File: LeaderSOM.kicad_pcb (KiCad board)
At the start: 4 copper layers, 61 x 50 mm, 108 parts, among them IC1 LP5912-3.3DRVR, IC2 TPS1120DR, J1 SWD, J10 SOMConnector, J11 CAN_Int, J2 USB_B_Micro, J4 Micro_SD_Card_Det, J5 CAN_In2, J6 CAN_Out2, J7 CarPowerConnector, J9 SOMConnector, Q1 PBSS4330X,135, Q2 SI7149ADP-T1-GE3, Q3 SI7149ADP-T1-GE3, SW1 Reset, SW2 BTN1, U1 MAX16914AUB/V+T, U3 CP2102N-A02-GQFN24, U4 ISO1044BD, U5 CDSOT23-T24CAN, U6 STM32F413RHTx, U8 ISO1044BD, U9 CDSOT23-T24CAN, Y2 8M

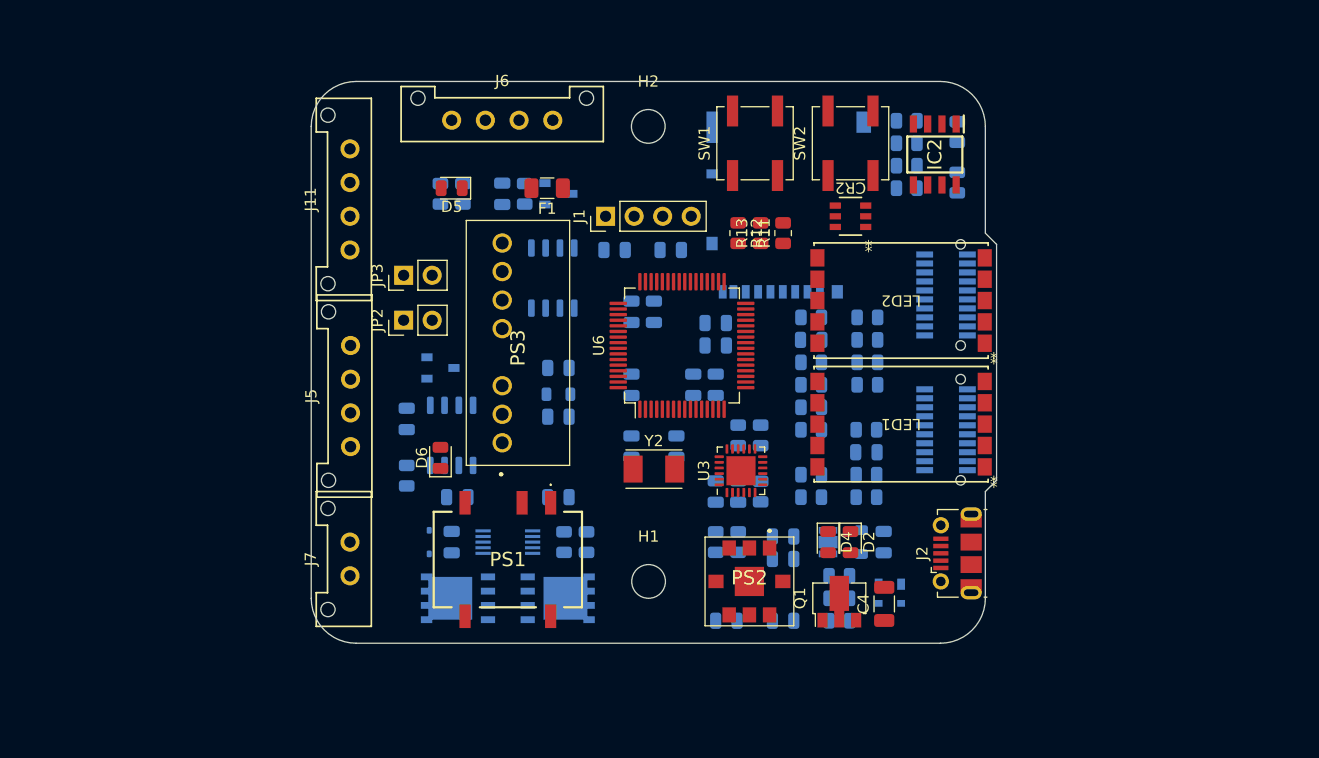
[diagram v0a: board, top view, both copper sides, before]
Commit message: hi lakshay
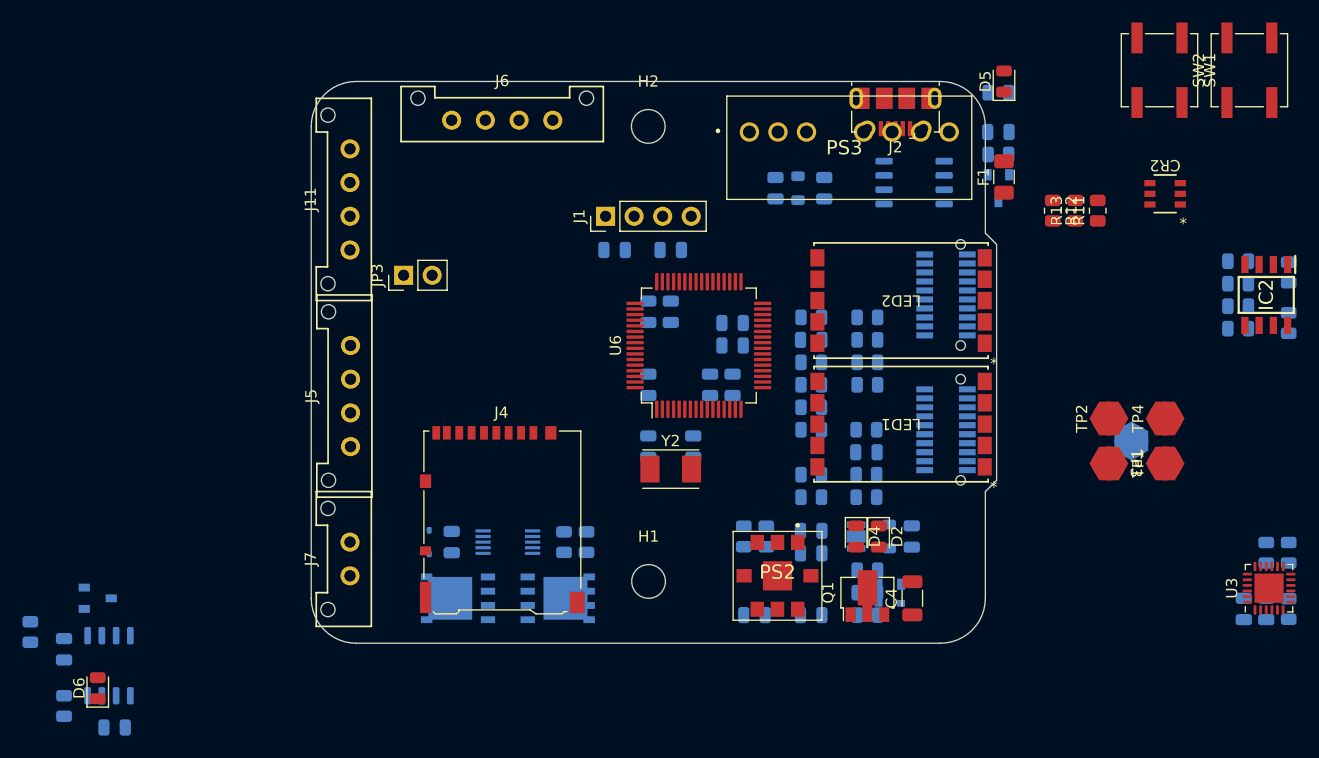
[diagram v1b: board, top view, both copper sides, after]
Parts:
- removed C3: 10uF, Capacitor_SMD:C_0805_2012Metric
- removed JP2: CAN_PWR Jumper, Connector_PinHeader_2.54mm:PinHeader_1x02_P2.54mm_Vertical
- removed PS1: 1769405141, UTSVT_Power:1769405141
- added TP1: +12V_TP, UTSVT_Special:TestPoint_HEX_3mmID, F.Cu at (166.0, 83.0)
- added TP2: +3V3_TP, UTSVT_Special:TestPoint_HEX_3mmID, F.Cu at (161.0, 79.0)
- added TP3: +5V_TP, UTSVT_Special:TestPoint_HEX_3mmID, F.Cu at (161.0, 83.0)
- added TP4: GND_TP, UTSVT_Special:TestPoint_HEX_3mmID, F.Cu at (166.0, 79.0)
- added TP6: GND_TP, UTSVT_Special:TestPoint_HEX_3mmID, B.Cu at (163.0, 81.0)
- J4: moved to F.Cu
- moved R22 53.4 mm to (65.0, 98.0)
- moved D5 50.1 mm to (151.7, 49.0), turned to 90 degrees
- moved R34 48.5 mm to (151.2, 50.0), turned to 180 degrees
- moved C18 48.1 mm to (173.0, 96.0)
- moved C19 48.1 mm to (175.0, 96.0)
- moved R5 48.1 mm to (177.0, 91.0)
- moved R6 48.1 mm to (175.0, 91.0)
- moved R8 48.1 mm to (177.0, 96.0)
- moved U3 48.1 mm to (175.2, 94.1)
- moved C10 44.5 mm to (151.2, 53.5), turned to 180 degrees
- moved R10 42.3 mm to (151.2, 55.5), turned to 180 degrees
- moved F1 40.7 mm to (151.7, 57.5), turned to 90 degrees
- moved J2 39.6 mm to (142.0, 51.7), turned to 180 degrees
- moved U5 39.2 mm to (151.2, 58.5), turned to -90 degrees
- moved J4 37.9 mm to (107.0, 88.0)
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
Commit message: u is for u n me
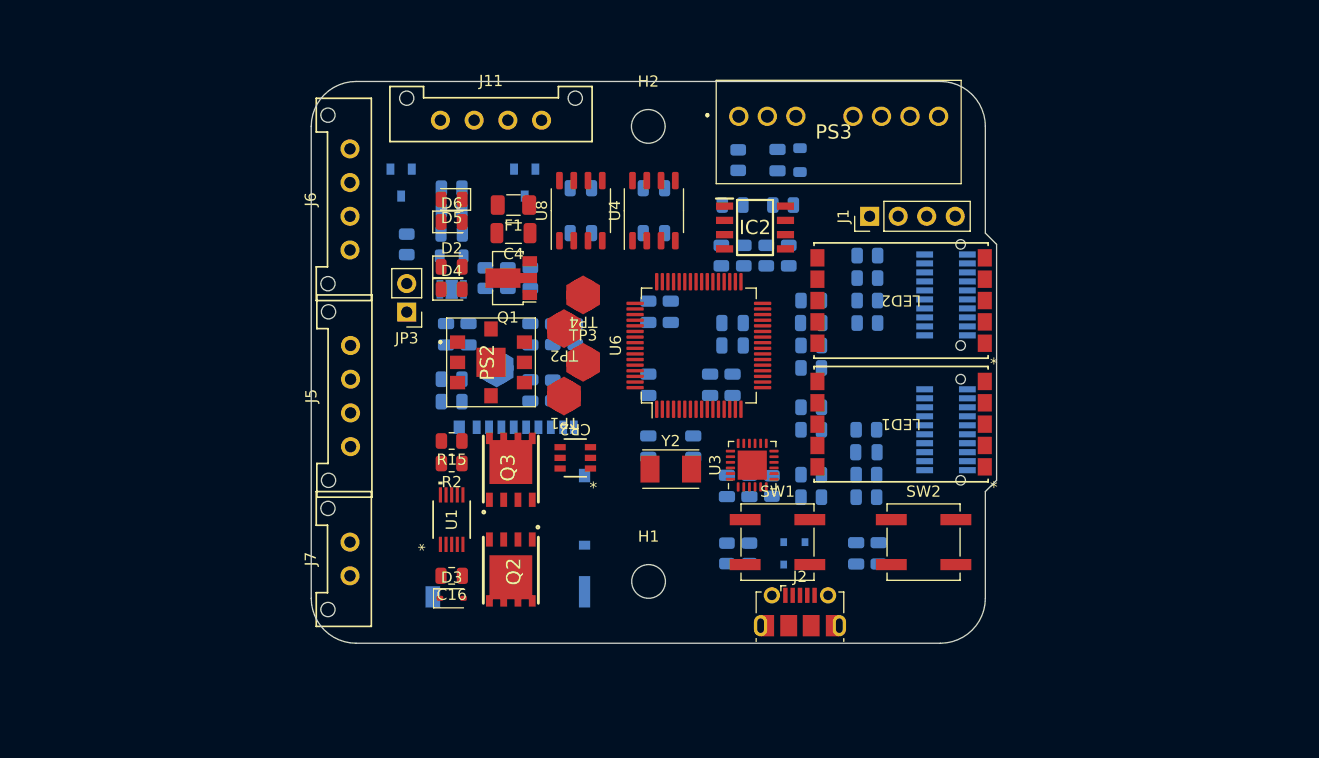
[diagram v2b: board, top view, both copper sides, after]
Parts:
- C16, D3, Q2, Q3, R15, R2, U1, U4, U8: moved to F.Cu
- J4, R11, R12, R13: moved to B.Cu
- moved C11 61.6 mm to (114.0, 58.5), turned to 0 degrees
- moved C8 60.5 mm to (114.0, 62.5), turned to 0 degrees
- moved U8 58.3 mm to (114.0, 60.5)
- moved CR2 57.5 mm to (113.5, 82.5)
- moved TP6 56.9 mm to (106.5, 74.5)
- moved R37 56.0 mm to (102.5, 60.5), turned to 0 degrees
- moved SW1 54.0 mm to (131.5, 90.0), turned to 0 degrees
- moved TP1 53.8 mm to (112.5, 77.0), turned to 180 degrees
- moved TP4 53.0 mm to (114.2, 68.0), turned to 180 degrees
- moved D6 52.1 mm to (102.5, 61.5), turned to 0 degrees
- moved SW2 51.0 mm to (144.5, 90.0), turned to 0 degrees
- moved D5 50.3 mm to (102.5, 59.5), turned to 180 degrees
- moved R17 49.9 mm to (127.5, 60.0), turned to 0 degrees
- moved R34 49.4 mm to (102.5, 58.5)
- moved C19 49.2 mm to (127.0, 85.0), turned to 90 degrees
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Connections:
- CR2 pad 1: /SPI1_CS -> /SPI1_SCK
- CR2 pad 3: /SPI1_MOSI -> /SPI1_MISO
- CR2 pad 4: /SPI1_SCK -> /SPI1_CS
- CR2 pad 6: /SPI1_MISO -> /SPI1_MOSI
- J4 pad 3: /SPI1_MISO -> /SPI1_MOSI
- R12 pad 1: /SPI1_MOSI -> /SPI1_MISO
